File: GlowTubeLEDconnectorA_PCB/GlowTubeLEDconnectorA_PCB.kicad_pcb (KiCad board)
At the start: 2 copper layers, 39.4 x 39.4 mm, 4 parts

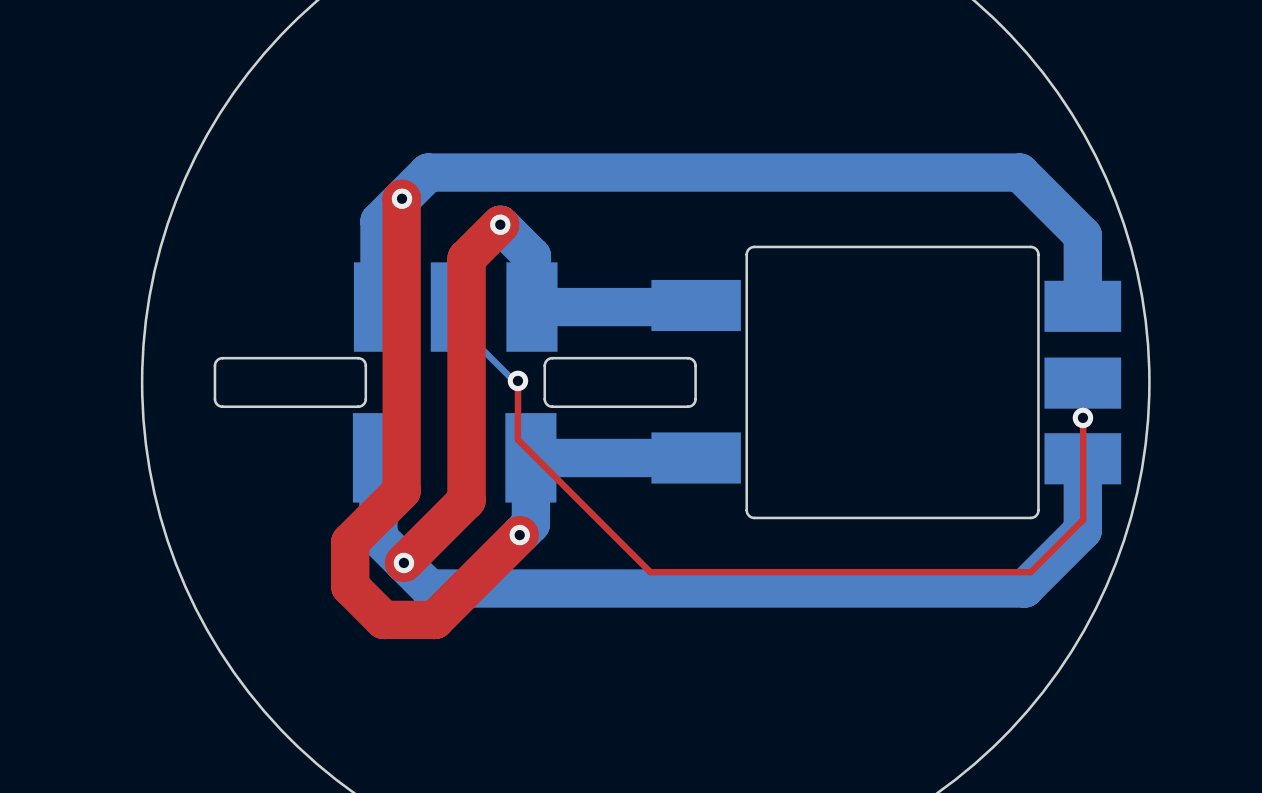
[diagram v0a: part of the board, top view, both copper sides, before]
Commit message: updated pcb design
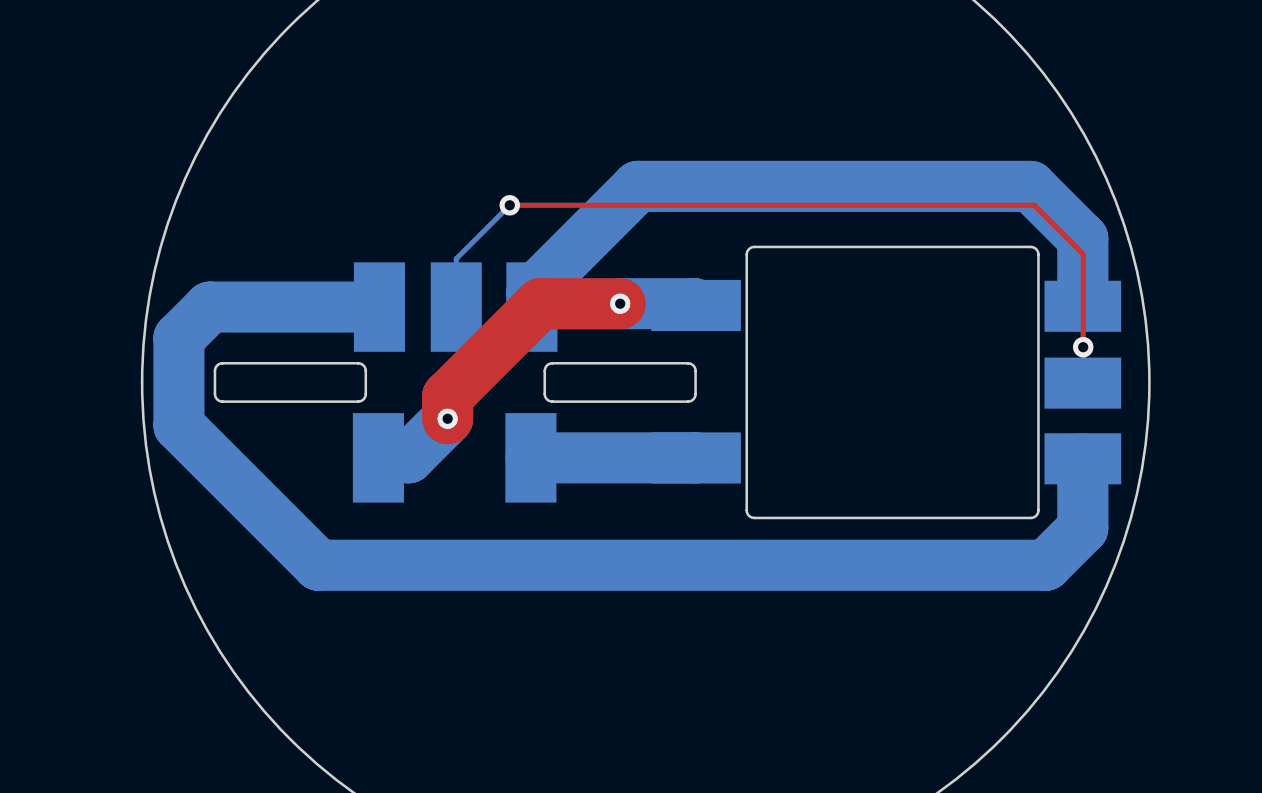
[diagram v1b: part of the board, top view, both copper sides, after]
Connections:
- LED1 pad 1: +5V -> GND
- LED1 pad 3: GND -> +5V
- LED3 pad 1: +5V -> GND
- LED3 pad 3: GND -> +5V
- LED4 pad 1: +5V -> GND
- LED4 pad 3: GND -> +5V
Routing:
- net +5V: track 69.7 -> 42.9 mm
- net LED1 DATA OUT: track 36.7 -> 33.1 mm
- net GND: track 60.2 -> 59.2 mm, vias 2 -> 0
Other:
- outline, holes or cut-outs redrawn
